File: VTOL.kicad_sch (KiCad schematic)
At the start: 36 parts, among them J10 I2C header, J5 USB_C_Receptacle_USB2.0_16P, J6 Conn_01x02_Pin, J7 Pi UART, J8 SEN66, J9 I2C header, SW1 RESET, SW2 BOOT, SW3 SW_SPDT, U4 ESP32-S3-WROOM-1, U5 USBLC6-2SC6, U6 AP7361C-33ER-13, U7 R-78E5.0-1.0

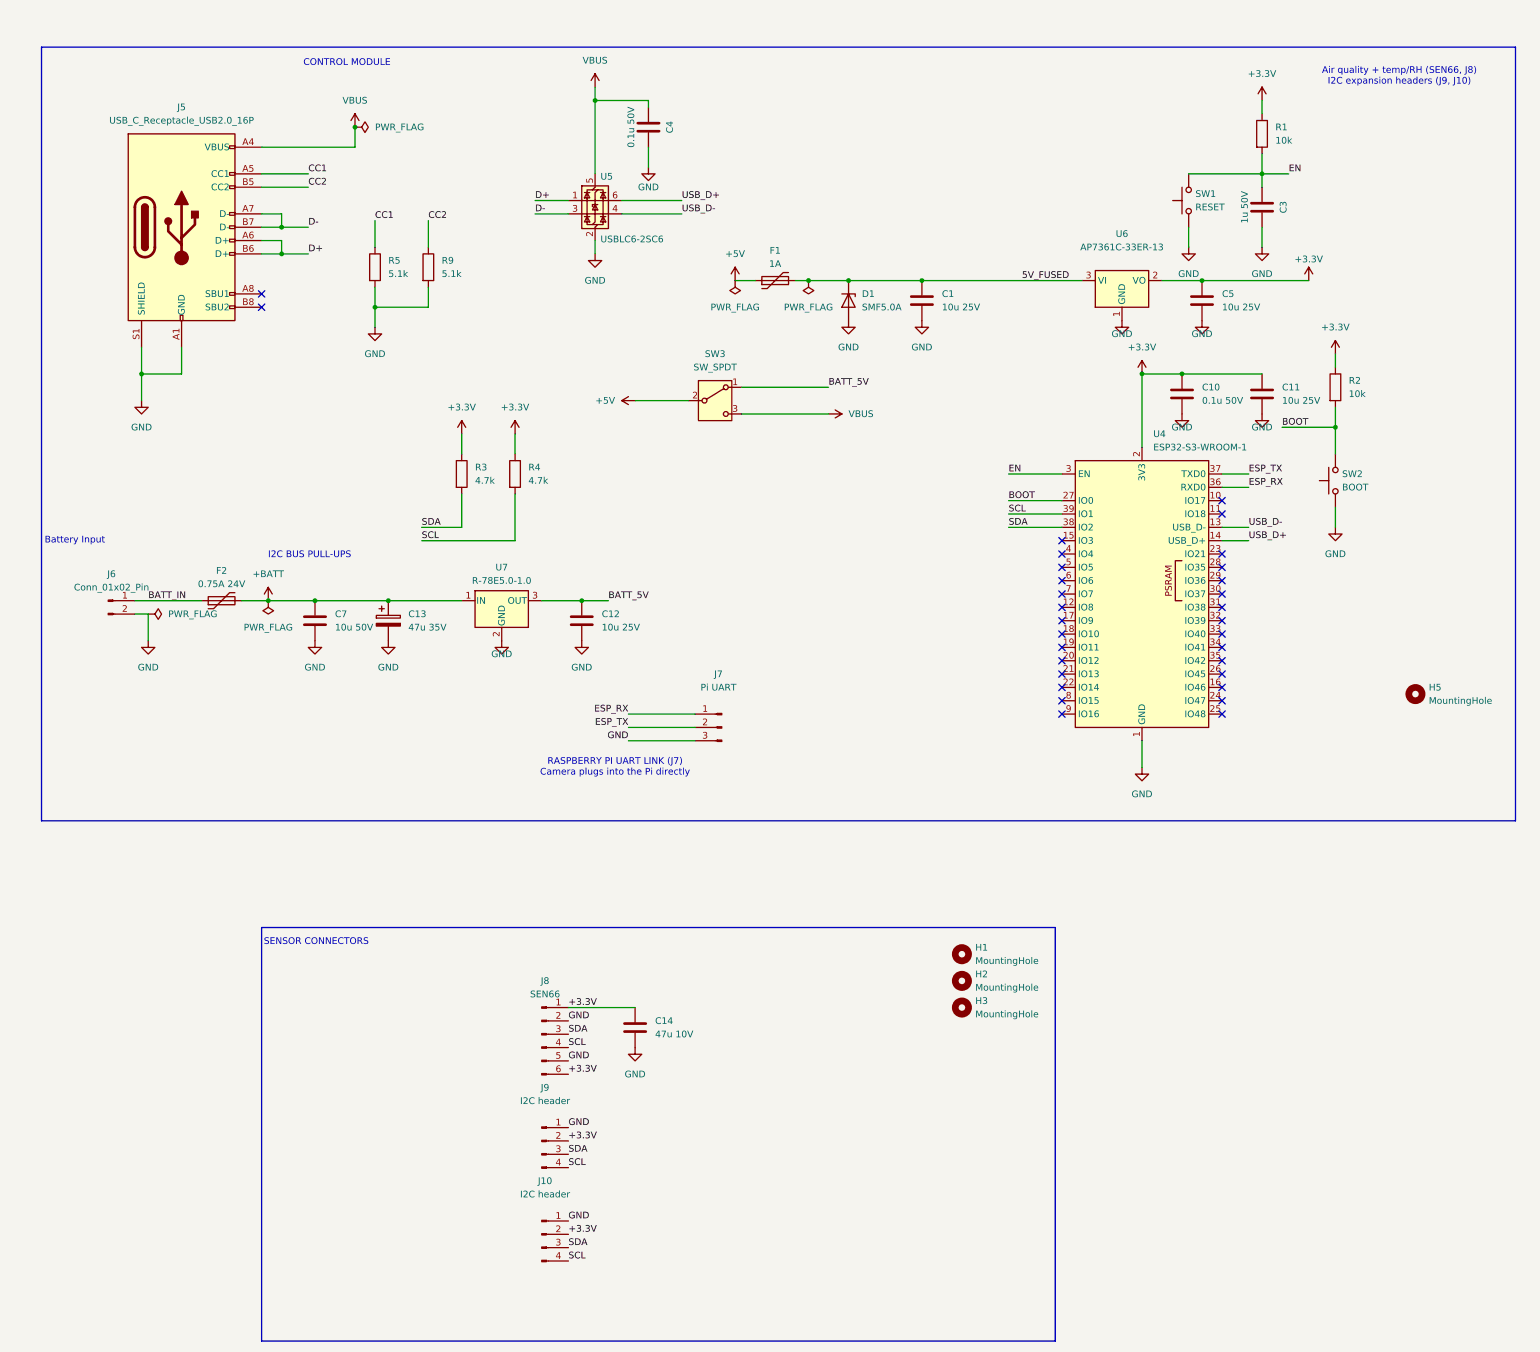
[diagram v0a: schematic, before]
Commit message: new schem
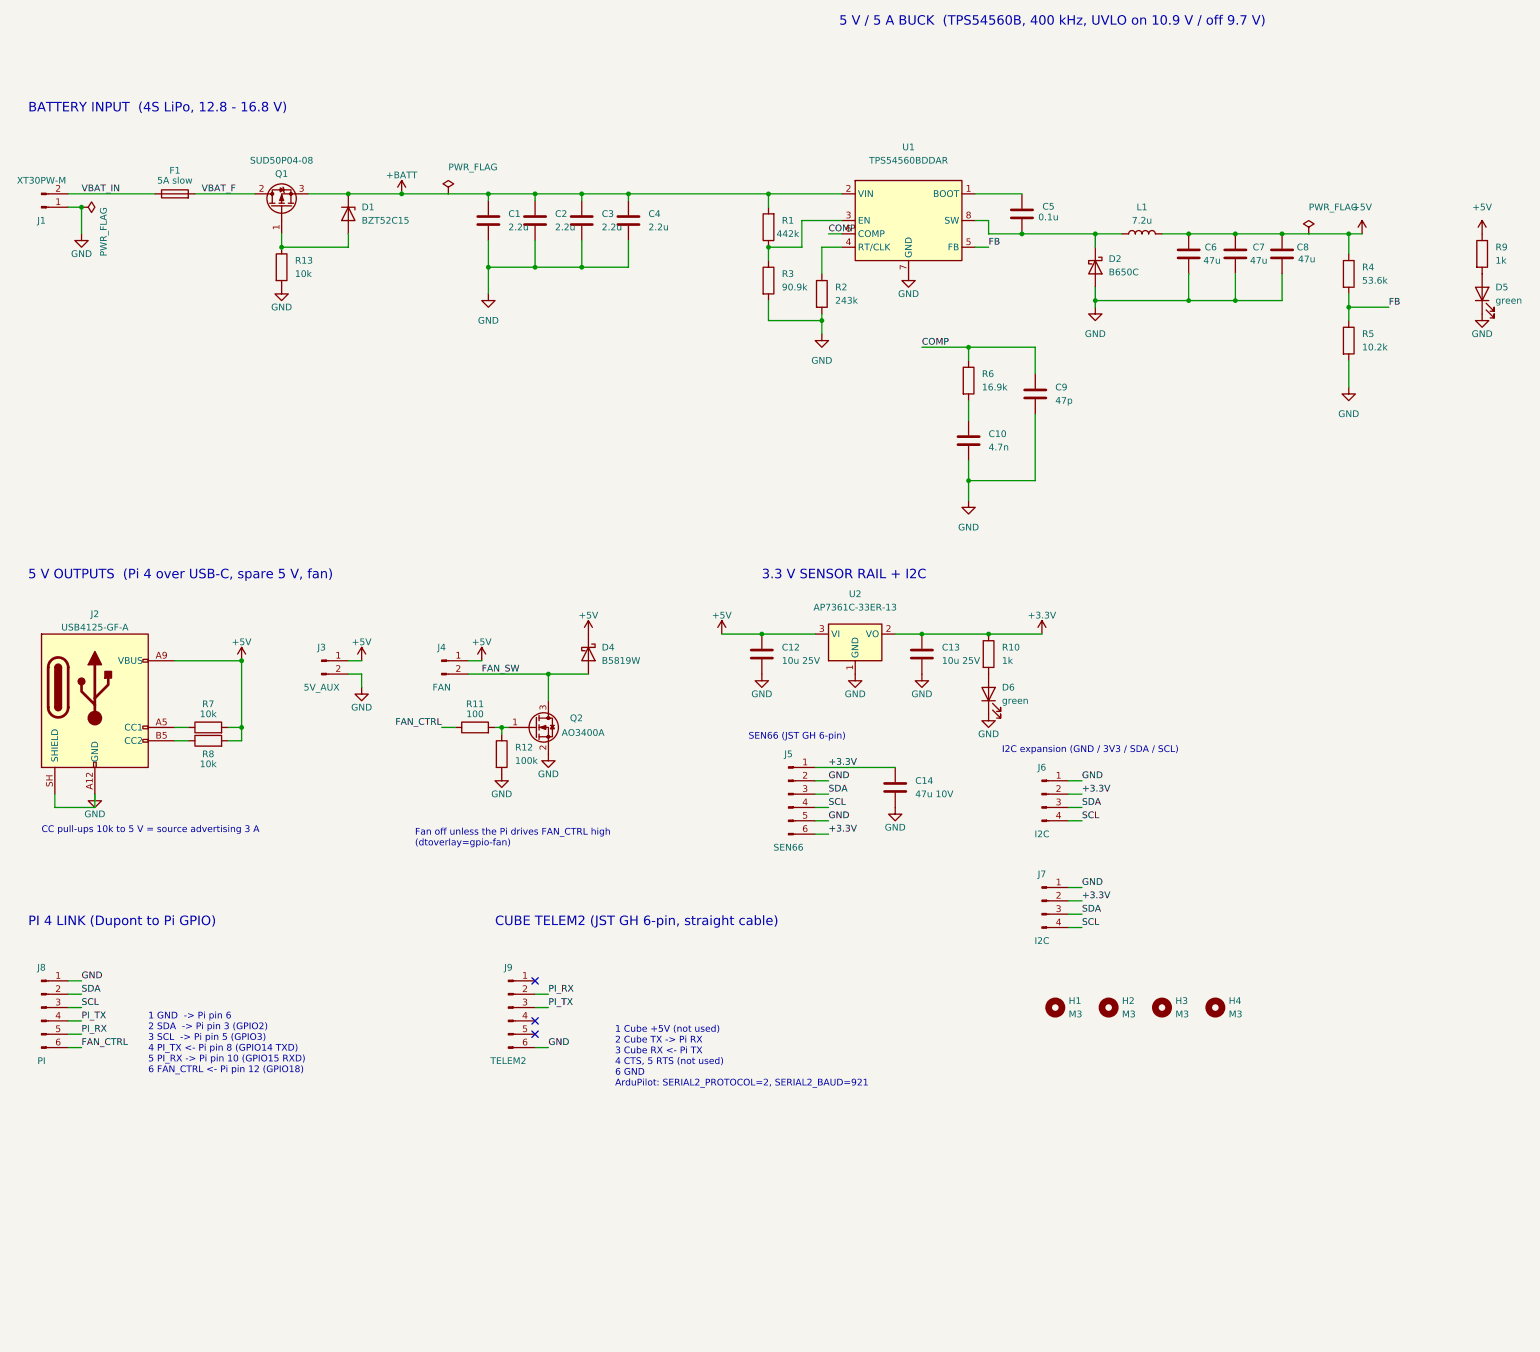
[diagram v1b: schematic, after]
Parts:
- removed C11: 10u 25V, Capacitor_SMD:C_0805_2012Metric_Pad1.18x1.45mm_HandSolder, symbol Device:C
- removed C13: 47u 35V, Capacitor_SMD:CP_Elec_6.3x5.8, symbol Device:C_Polarized
- removed D1: SMF5.0A, Diode_SMD:D_SOD-123F, symbol Diode:PTVS5V0Z1USK
- removed F1: 1A, Fuse:Fuse_1206_3216Metric_Pad1.42x1.75mm_HandSolder, symbol Device:Polyfuse
- removed F2: 0.75A 24V, Fuse:Fuse_1812_4532Metric_Pad1.30x3.40mm_HandSolder, symbol Device:Polyfuse
- removed H5: MountingHole, MountingHole:MountingHole_3.2mm_M3_Pad_Via, symbol Mechanical:MountingHole
- removed J10, J9: I2C header, Connector_PinHeader_2.54mm:PinHeader_1x04_P2.54mm_Vertical, symbol Connector:Conn_01x04_Pin
- removed J5: USB_C_Receptacle_USB2.0_16P, VTOL_parts:USB_C_Receptacle_GCT_USB4105-GF-A_16P_TopMnt_Horizontal_S1, symbol Connector:USB_C_Receptacle_USB2.0_16P
- removed J6: Conn_01x02_Pin, Connector_JST:JST_PH_S2B-PH-K_1x02_P2.00mm_Horizontal, symbol Connector:Conn_01x02_Pin
- removed J7: Pi UART, Connector_PinHeader_2.54mm:PinHeader_1x03_P2.54mm_Vertical, symbol Connector:Conn_01x03_Pin
- removed SW1: RESET, Button_Switch_SMD:SW_SPST_PTS645Sx43SMTR92, symbol Switch:SW_Push
- removed SW2: BOOT, Button_Switch_SMD:SW_SPST_PTS645Sx43SMTR92, symbol Switch:SW_Push
- removed SW3: SW_SPDT, VTOL_parts:SW_Slide_SPDT_RightAngle_CK_1101M2S3AQE2, symbol Switch:SW_SPDT
- removed U4: ESP32-S3-WROOM-1, VTOL_parts:ESP32-S3-WROOM-1_Via0.3mm, symbol RF_Module:ESP32-S3-WROOM-1
- removed U5: USBLC6-2SC6, Package_TO_SOT_SMD:SOT-23-6, symbol Power_Protection:USBLC6-2SC6
- removed U6: AP7361C-33ER-13, Package_TO_SOT_SMD:SOT-223-3_TabPin2, symbol Regulator_Linear:AMS1117-3.3
- removed U7: R-78E5.0-1.0, Converter_DCDC:Converter_DCDC_RECOM_R-78E-0.5_THT, symbol Converter_DCDC:R-78E5.0-1.0
- added C13: 10u 25V, Capacitor_SMD:C_0805_2012Metric_Pad1.18x1.45mm_HandSolder, symbol Device:C
- added C2: 2.2u, Capacitor_SMD:C_1206_3216Metric_Pad1.33x1.80mm_HandSolder, symbol Device:C
- added C6, C8: 47u, Capacitor_SMD:C_1206_3216Metric_Pad1.33x1.80mm_HandSolder, symbol Device:C
- added C9: 47p, Capacitor_SMD:C_0603_1608Metric_Pad1.08x0.95mm_HandSolder, symbol Device:C
- added D1: BZT52C15, Diode_SMD:D_SOD-123, symbol Device:D_Zener
- added D2: B650C, Diode_SMD:D_SMC, symbol Device:D_Schottky
- added D4: B5819W, Diode_SMD:D_SOD-123, symbol Device:D_Schottky
- added D5, D6: green, LED_SMD:LED_0603_1608Metric_Pad1.05x0.95mm_HandSolder, symbol Device:LED
- added F1: 5A slow, Fuse:Fuse_Littelfuse-NANO2-451_453, symbol Device:Fuse
- added H4: M3, MountingHole:MountingHole_3.2mm_M3, symbol Mechanical:MountingHole
- added J1: XT30PW-M, Connector_AMASS:AMASS_XT30PW-M_1x02_P2.50mm_Horizontal, symbol Connector:Conn_01x02_Pin
- added J2: USB4125-GF-A, Connector_USB:USB_C_Receptacle_GCT_USB4125-xx-x_6P_TopMnt_Horizontal, symbol Connector:USB_C_Receptacle_PowerOnly_6P
- added J3: 5V_AUX, Connector_PinHeader_2.54mm:PinHeader_1x02_P2.54mm_Vertical, symbol Connector:Conn_01x02_Pin
- added J4: FAN, Connector_PinHeader_2.54mm:PinHeader_1x02_P2.54mm_Vertical, symbol Connector:Conn_01x02_Pin
- added J5: SEN66, Connector_JST:JST_GH_BM06B-GHS-TBT_1x06-1MP_P1.25mm_Vertical, symbol Connector:Conn_01x06_Pin
- added J6, J7: I2C, Connector_PinHeader_2.54mm:PinHeader_1x04_P2.54mm_Vertical, symbol Connector:Conn_01x04_Pin
- added J9: TELEM2, Connector_JST:JST_GH_BM06B-GHS-TBT_1x06-1MP_P1.25mm_Vertical, symbol Connector:Conn_01x06_Pin
- added L1: 7.2u, Inductor_SMD:L_Coilcraft_XAL7070-XXX, symbol Device:L
- added Q1: SUD50P04-08, Package_TO_SOT_SMD:TO-252-2, symbol Transistor_FET:SUD50P04-08
- added Q2: AO3400A, Package_TO_SOT_SMD:SOT-23, symbol Transistor_FET:AO3400A
- added R10: 1k, Resistor_SMD:R_0603_1608Metric_Pad0.98x0.95mm_HandSolder, symbol Device:R
- added R11: 100, Resistor_SMD:R_0603_1608Metric_Pad0.98x0.95mm_HandSolder, symbol Device:R
- added R12: 100k, Resistor_SMD:R_0603_1608Metric_Pad0.98x0.95mm_HandSolder, symbol Device:R
- added R13, R7, R8: 10k, Resistor_SMD:R_0603_1608Metric_Pad0.98x0.95mm_HandSolder, symbol Device:R
- added R6: 16.9k, Resistor_SMD:R_0603_1608Metric_Pad0.98x0.95mm_HandSolder, symbol Device:R
- added U1: TPS54560BDDAR, Package_SO:Texas_R-PDSO-G8_EP2.95x4.9mm_Mask2.4x3.1mm_ThermalVias, symbol Regulator_Switching:TPS54560BDDA
- added U2: AP7361C-33ER-13, Package_TO_SOT_SMD:SOT-223-3_TabPin2, symbol Regulator_Linear:AMS1117-3.3
- C1: value 10u 25V -> 2.2u; footprint Capacitor_SMD:C_0805_2012Metric_Pad1.18x1.45mm_HandSolder -> Capacitor_SMD:C_1206_3216Metric_Pad1.33x1.80mm_HandSolder
- C10: value 0.1u 50V -> 4.7n
- C12: MPN (none) -> Samsung CL21A106KAQNNNE
- C14: MPN (none) -> Murata GRM31CR61A476KE15L
- C3: value 1u 50V -> 2.2u; footprint Capacitor_SMD:C_0603_1608Metric_Pad1.08x0.95mm_HandSolder -> Capacitor_SMD:C_1206_3216Metric_Pad1.33x1.80mm_HandSolder
- C4: value 0.1u 50V -> 2.2u; footprint Capacitor_SMD:C_0603_1608Metric_Pad1.08x0.95mm_HandSolder -> Capacitor_SMD:C_1206_3216Metric_Pad1.33x1.80mm_HandSolder
- C5: value 10u 25V -> 0.1u; footprint Capacitor_SMD:C_0805_2012Metric_Pad1.18x1.45mm_HandSolder -> Capacitor_SMD:C_0603_1608Metric_Pad1.08x0.95mm_HandSolder
- C7: value 10u 50V -> 47u
- H1, H2, H3: value MountingHole -> M3; footprint MountingHole:MountingHole_3.2mm_M3_Pad_Via -> MountingHole:MountingHole_3.2mm_M3; now in the parts list
- J8: value SEN66 -> PI; footprint Connector_JST:JST_GH_BM06B-GHS-TBT_1x06-1MP_P1.25mm_Vertical -> Connector_PinHeader_2.54mm:PinHeader_1x06_P2.54mm_Vertical; MPN (none) -> 2.54 mm header
- R1: value 10k -> 442k
- R2: value 10k -> 243k
- R3: value 4.7k -> 90.9k
- R4: value 4.7k -> 53.6k
- R5: value 5.1k -> 10.2k
- R9: value 5.1k -> 1k; MPN (none) -> Yageo RC0603FR-071KL
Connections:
- net 5V_FUSED is gone; now on net +BATT: C1.1
- net BATT_5V is gone; now on net +5V: C12.1
- net BOOT is gone; now on net GND: R2.2
- net CC2 is gone; now on net +5V: R9.1
- net VBUS is gone; now on net GND: C4.2
- net +3.3V: now also C13.1, J5.1 (Pin_1), J5.6 (Pin_6), J6.2 (Pin_2), J7.2 (Pin_2), R10.1, U2.2 (VO); no longer C10.1, C5.1, J8.1 (Pin_1), J8.6 (Pin_6), R1.1, R2.1, R3.1, R4.1
- net +5V: now also C7.1, R4.1, C6.1, C8.1, D4.1 (K), J2.A9 (VBUS), J2.B9 (VBUS), J3.1 (Pin_1), J4.1 (Pin_1), L1.2, R7.2, R8.2, U2.3 (VI)
- net +BATT: now also C3.1, C4.1, R1.2, C2.1, D1.1 (K), Q1.3 (S), U1.2 (VIN); no longer C7.1
- net GND: now also C3.2, J8.1 (Pin_1), R3.2, C13.2, C2.2, C6.2, C8.2, C9.2, D2.2 (A), D5.1 (K), D6.1 (K), J1.1 (Pin_1), J2.A12 (GND), J2.B12 (GND), J2.SH (SHIELD), J3.2 (Pin_2), J5.2 (Pin_2), J5.5 (Pin_5), J6.1 (Pin_1), J7.1 (Pin_1), J9.6 (Pin_6), Q2.2 (S), R12.2, R13.2, U1.7 (GND), U1.9 (GND), U2.1 (GND); no longer C3.1, C4.1, C5.2, J8.2 (Pin_2), J8.5 (Pin_5), R9.2
- net SCL: now also J8.3 (Pin_3), J5.4 (Pin_4), J6.4 (Pin_4), J7.4 (Pin_4); no longer J8.4 (Pin_4), R4.2
- net SDA: now also J8.2 (Pin_2), J5.3 (Pin_3), J6.3 (Pin_3), J7.3 (Pin_3); no longer J8.3 (Pin_3), R3.2
- net CC1 renamed FB
- net FB: now also R4.2, U1.5 (FB)
- removed net EN: C3.2, R1.2
- new net: C5.2, U1.1 (BOOT)
- new net: R1.1, R3.1, U1.3 (EN)
- new net: R2.1, U1.4 (RT/CLK)
- new net: C5.1, D2.1 (K), L1.1, U1.8 (SW)
- new net: C10.1, R6.2
- new net: D1.2 (A), Q1.1 (G), R13.1
- new net: Q2.1 (G), R11.2, R12.1
- new net: D5.2 (A), R9.2
- new net: J2.A5 (CC1), R7.1
- new net: J2.B5 (CC2), R8.1
- new net: D6.2 (A), R10.2
- new net COMP: C9.1, R6.1, U1.6 (COMP)
- new net FAN_CTRL: J8.6 (Pin_6), R11.1
- new net FAN_SW: D4.2 (A), J4.2 (Pin_2), Q2.3 (D)
- new net PI_RX: J8.5 (Pin_5), J9.2 (Pin_2)
- new net PI_TX: J8.4 (Pin_4), J9.3 (Pin_3)
- new net VBAT_F: F1.2, Q1.2 (D)
- new net VBAT_IN: F1.1, J1.2 (Pin_2)
- no-connect marks 31 -> 3
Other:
- note added: "1 Cube +5V (not used) 2 Cube TX -> Pi RX 3 Cube RX <- Pi TX 4 CTS, 5 RTS (not used) 6 GND ArduPilot: SERIAL2_PROTOCOL=2, SERIAL2_BAUD=921"
- note added: "1 GND -> Pi pin 6 2 SDA -> Pi pin 3 (GPIO2) 3 SCL -> Pi pin 5 (GPIO3) 4 PI_TX <- Pi pin 8 (GPIO14 TXD) 5 PI_RX -> Pi pin 10 (GPIO15 RXD) 6 FAN_CTRL <- Pi pin 12 (GPIO18)"
- note added: "3.3 V SENSOR RAIL + I2C"
- note added: "5 V / 5 A BUCK (TPS54560B, 400 kHz, UVLO on 10.9 V / off 9.7 V)"
- note added: "5 V OUTPUTS (Pi 4 over USB-C, spare 5 V, fan)"
- note added: "BATTERY INPUT (4S LiPo, 12.8 - 16.8 V)"
- note added: "CC pull-ups 10k to 5 V = source advertising 3 A"
- note added: "CUBE TELEM2 (JST GH 6-pin, straight cable)"
- note added: "Fan off unless the Pi drives FAN_CTRL high (dtoverlay=gpio-fan)"
- note added: "I2C expansion (GND / 3V3 / SDA / SCL)"
- note added: "PI 4 LINK (Dupont to Pi GPIO)"
- note added: "SEN66 (JST GH 6-pin)"
- note removed: "Air quality + temp/RH (SEN66, J8) I2C expansion headers (J9, J10)"
- note removed: "Battery Input"
- note removed: "CONTROL MODULE"
- note removed: "I2C BUS PULL-UPS"
- note removed: "RASPBERRY PI UART LINK (J7) Camera plugs into the Pi directly"
- note removed: "SENSOR CONNECTORS"
- title: Module Control Board -> Pi Power and Sensor Board
